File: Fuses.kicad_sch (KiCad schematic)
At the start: 24 parts, among them J2 Conn_01x02_Female, J3 Conn_01x02_Female, J4 Conn_01x02_Female, J5 Conn_01x02_Female, J6 Conn_01x02_Female, J7 Conn_01x02_Female, J8 Conn_01x02_Female, J9 Conn_01x02_Female

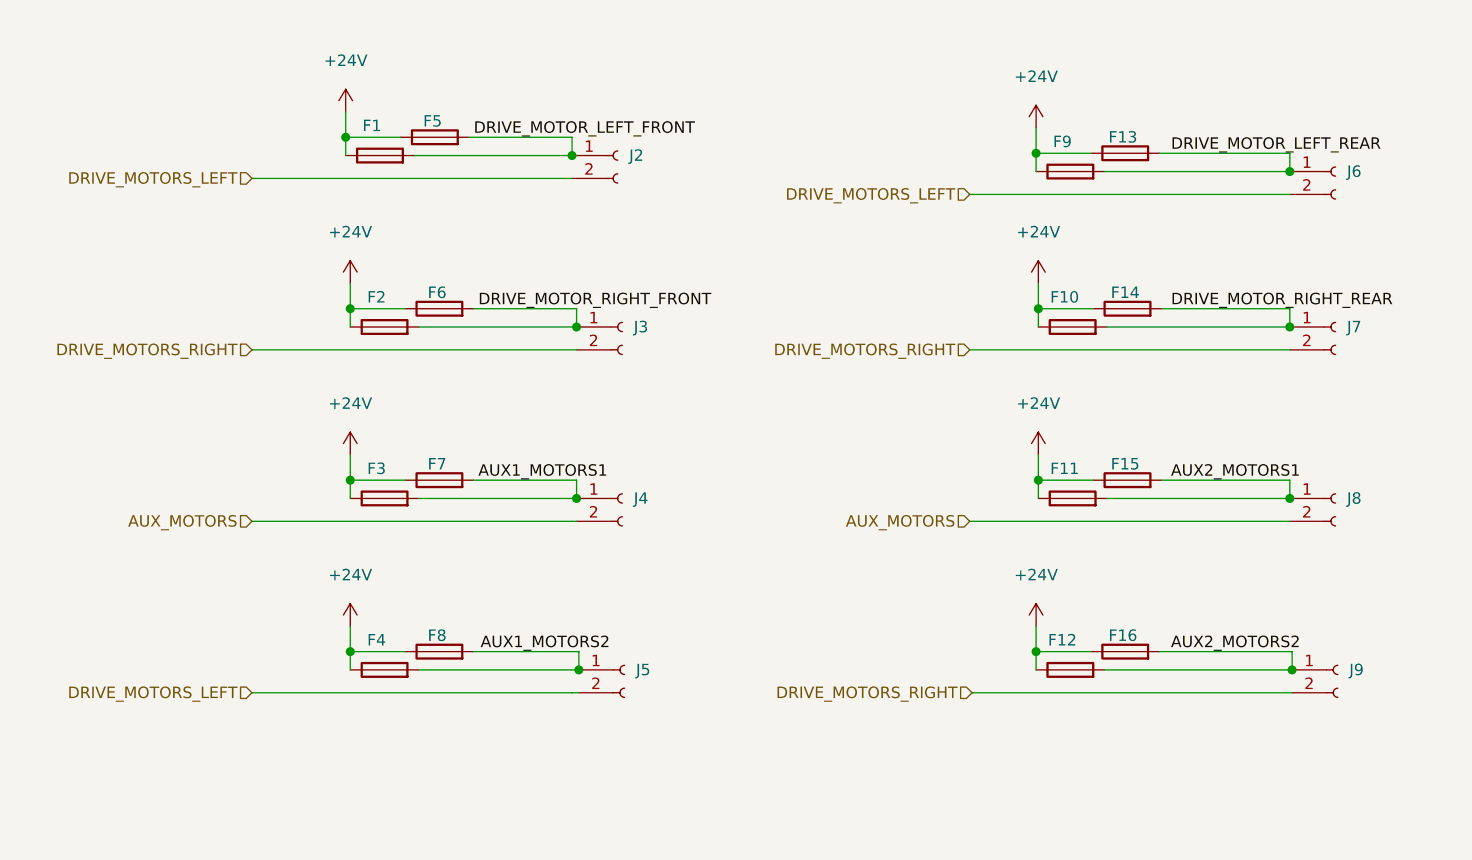
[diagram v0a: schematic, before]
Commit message: Updated according to requirements
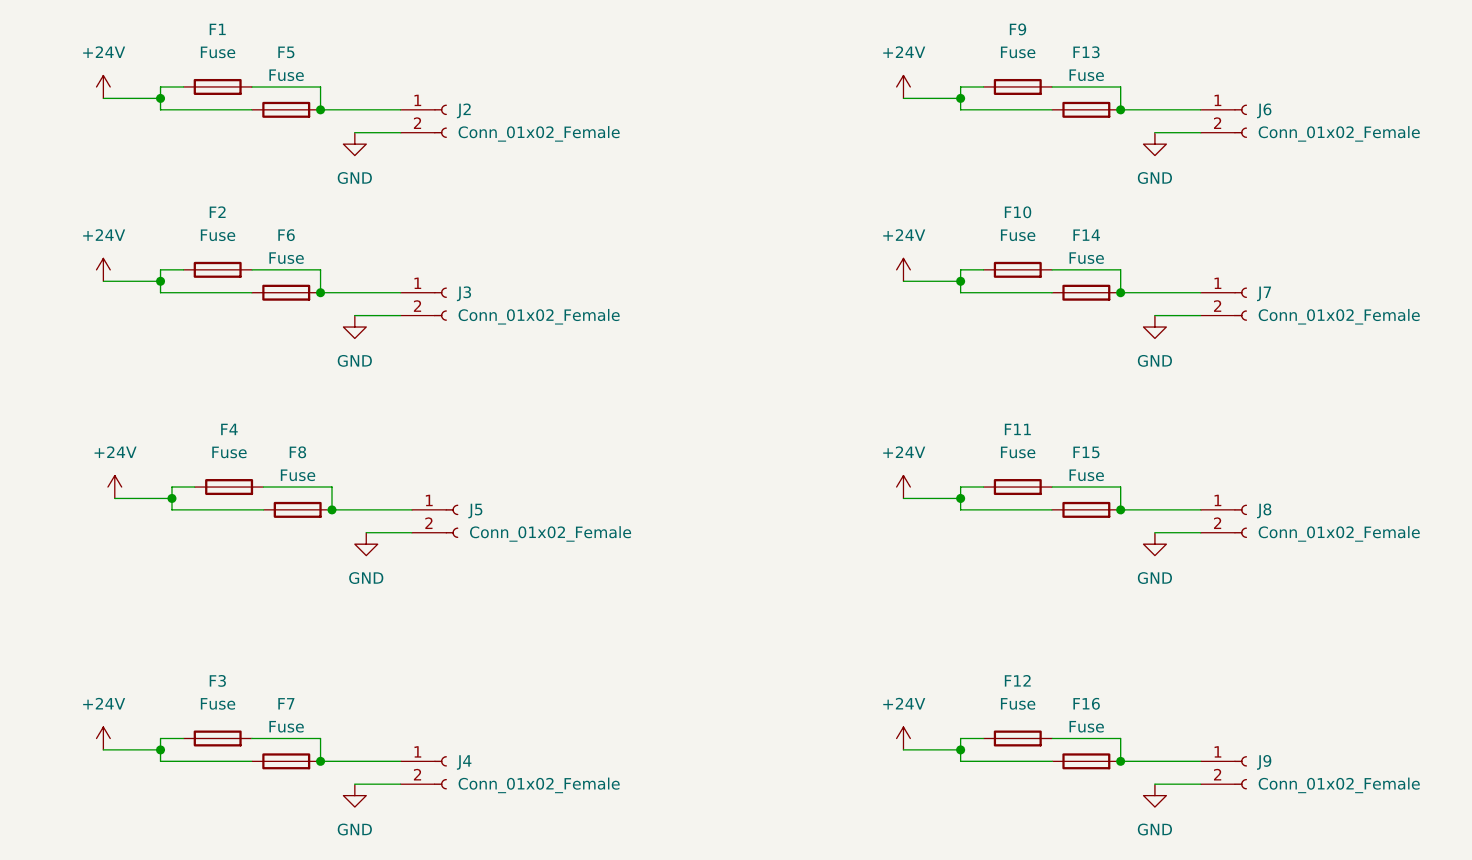
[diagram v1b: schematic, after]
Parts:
- J2, J3, J4, J5, J6, J7, J8, J9: footprint Connector_JST:JST_XH_B2B-XH-AM_1x02_P2.50mm_Vertical -> Connector_JST:JST_XH_B2B-XH-A_1x02_P2.50mm_Vertical
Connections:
- net DRIVE_MOTORS_LEFT is gone; now on net GND: J2.2 (Pin_2), J5.2 (Pin_2), J6.2 (Pin_2)
- net DRIVE_MOTORS_RIGHT is gone; now on net GND: J3.2 (Pin_2), J7.2 (Pin_2), J9.2 (Pin_2)
- net AUX1_MOTORS1: no longer names the net of F3.2, F7.2, J4.1 (Pin_1)
- net AUX1_MOTORS2: no longer names the net of F4.2, F8.2, J5.1 (Pin_1)
- net AUX2_MOTORS1: no longer names the net of F11.2, F15.2, J8.1 (Pin_1)
- net AUX2_MOTORS2: no longer names the net of F12.2, F16.2, J9.1 (Pin_1)
- net AUX_MOTORS renamed GND
- net DRIVE_MOTOR_LEFT_FRONT: no longer names the net of F1.2, F5.2, J2.1 (Pin_1)
- net DRIVE_MOTOR_LEFT_REAR: no longer names the net of F13.2, F9.2, J6.1 (Pin_1)
- net DRIVE_MOTOR_RIGHT_FRONT: no longer names the net of F2.2, F6.2, J3.1 (Pin_1)
- net DRIVE_MOTOR_RIGHT_REAR: no longer names the net of F10.2, F14.2, J7.1 (Pin_1)
